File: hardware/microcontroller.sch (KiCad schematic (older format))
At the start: 10 parts, among them J1 Conn_02x05_Odd_Even, U1 ESP-WROOM-32

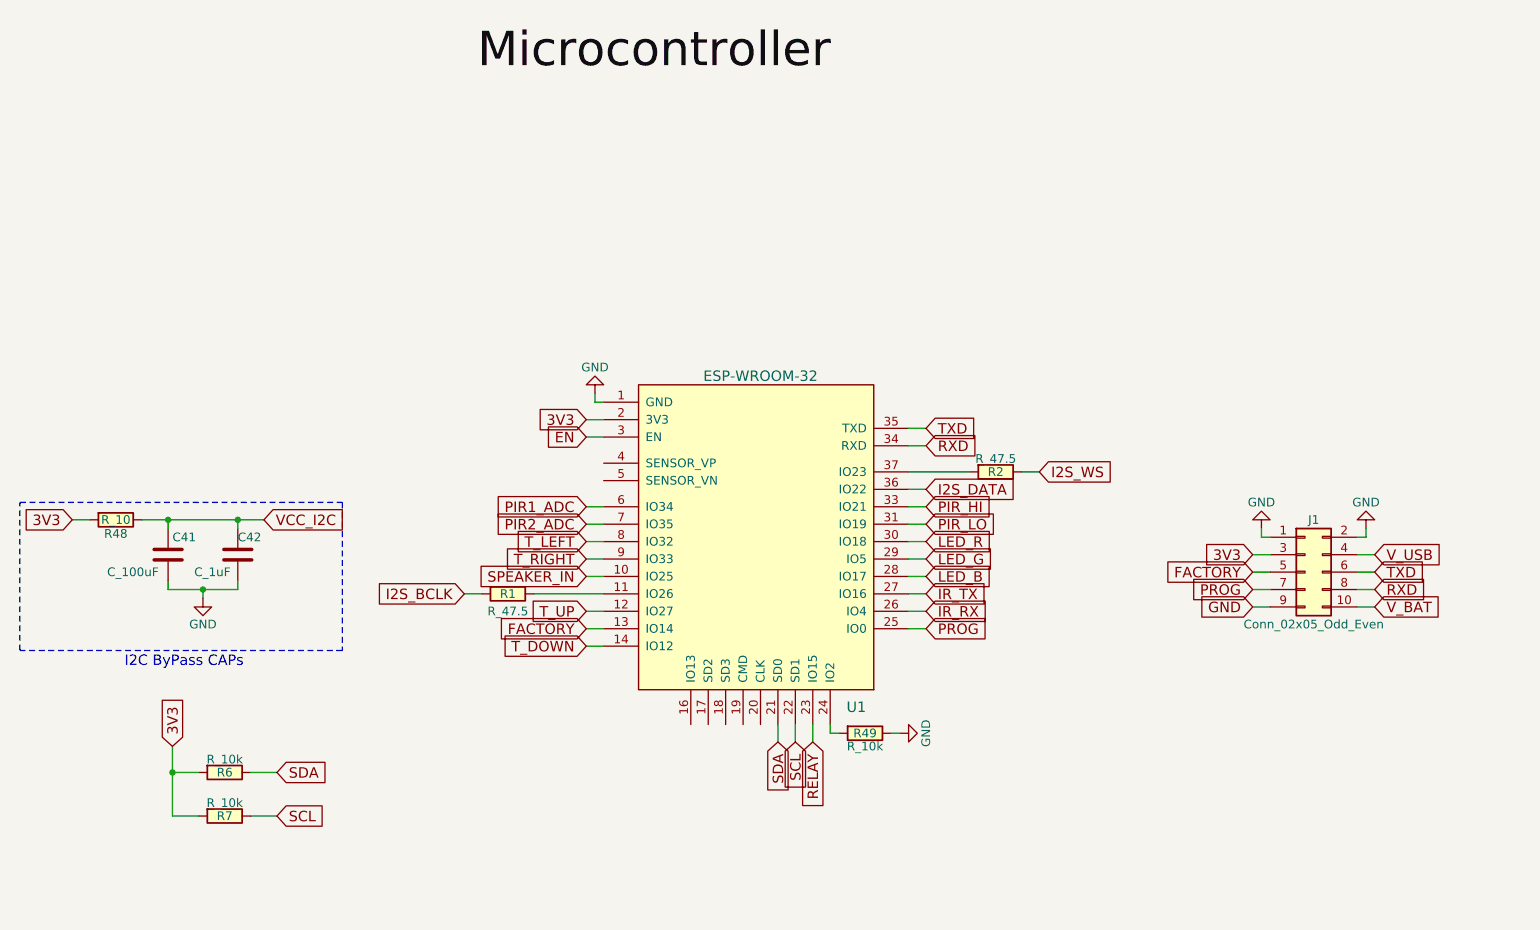
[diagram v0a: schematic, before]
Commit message: update
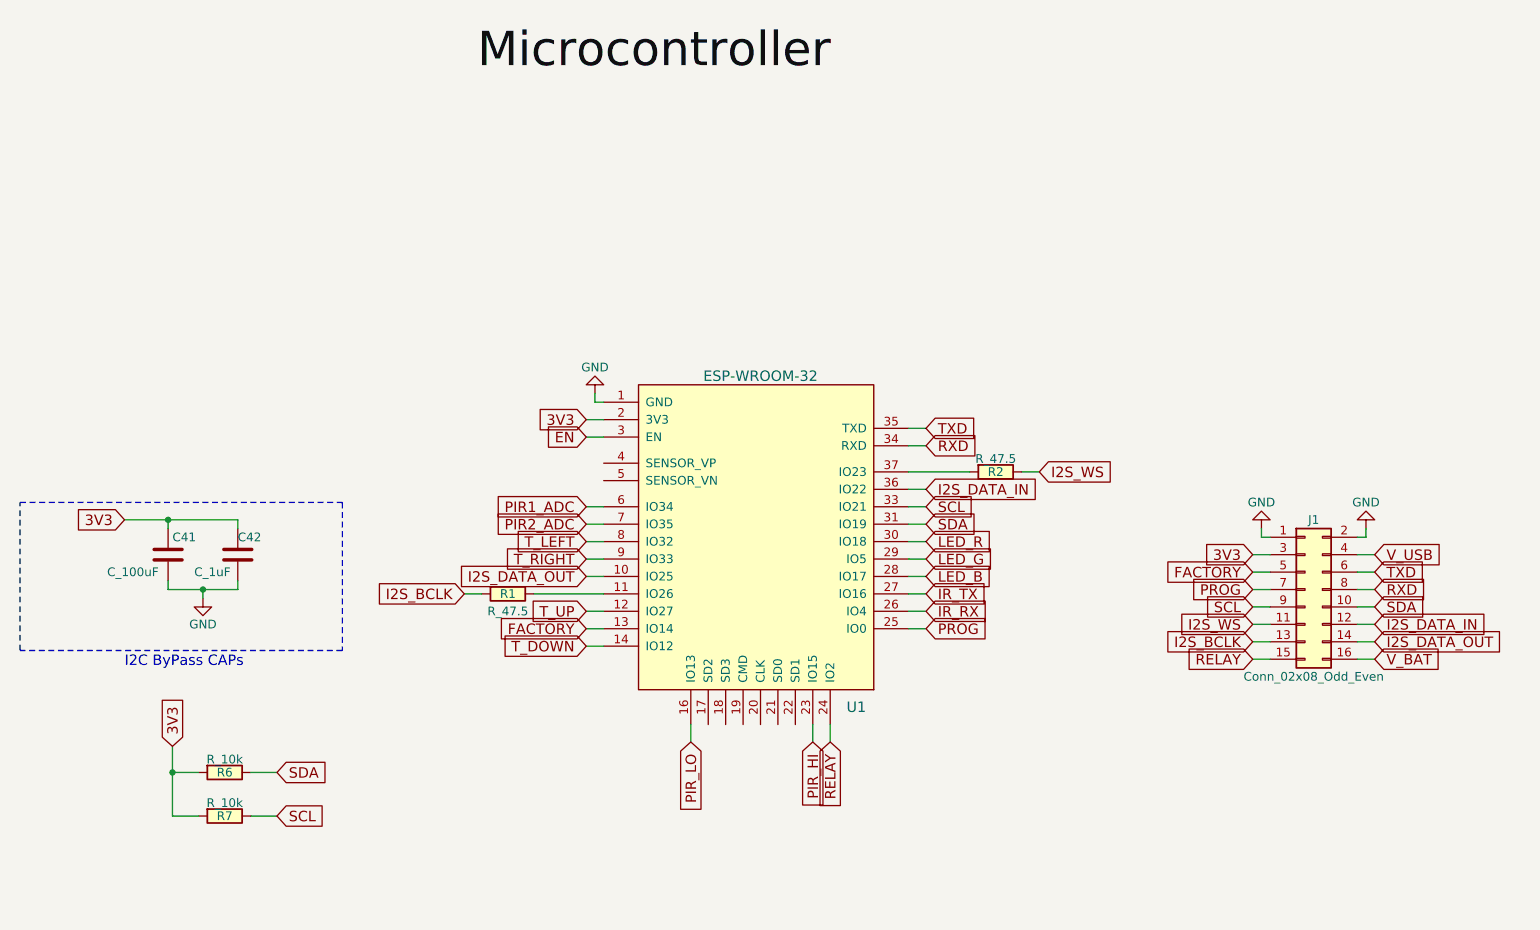
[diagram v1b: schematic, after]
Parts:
- removed J1: Conn_02x05_Odd_Even, Pin_Headers:Pin_Header_Straight_2x05_Pitch2.54mm, symbol Conn_02x05_Odd_Even
- removed R48: R_10, Resistors_SMD:R_0603, symbol R_10
- removed R49: R_10k, Resistors_SMD:R_0603, symbol R_10k
- added J1: Conn_02x08_Odd_Even, Pin_Headers:Pin_Header_Straight_2x08_Pitch2.54mm, symbol Conn_02x08_Odd_Even
- C41: footprint Capacitors_SMD:C_1206 -> Capacitors_SMD:C_1206_HandSoldering
- C42: footprint Capacitors_SMD:C_0603 -> Capacitors_SMD:C_0603_HandSoldering
- R1, R2, R6, R7: footprint Resistors_SMD:R_0603 -> Resistors_SMD:R_0603_HandSoldering
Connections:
- net VCC_I2C is gone; now on net 3V3: C41.1, C42.1
- net 3V3: now also J1.3 (Pin_3)
- net FACTORY: now also J1.5 (Pin_5)
- net GND: now also J1.1 (Pin_1), J1.2 (Pin_2)
- net I2S_BCLK: now also J1.13 (Pin_13)
- net I2S_WS: now also J1.11 (Pin_11)
- net PIR_HI: now also U1.23 (IO15); no longer U1.33 (IO21)
- net PIR_LO: now also U1.16 (IO13); no longer U1.31 (IO19)
- net PROG: now also J1.7 (Pin_7)
- net RELAY: now also U1.24 (IO2), J1.15 (Pin_15); no longer U1.23 (IO15)
- net RXD: now also J1.8 (Pin_8)
- net SCL: now also U1.33 (IO21), J1.9 (Pin_9); no longer U1.22 (SD1)
- net SDA: now also U1.31 (IO19), J1.10 (Pin_10); no longer U1.21 (SD0)
- net TXD: now also J1.6 (Pin_6)
- net V_BAT: now also J1.16 (Pin_16)
- net V_USB: now also J1.4 (Pin_4)
- net I2S_DATA renamed I2S_DATA_IN
- net I2S_DATA_IN: now also J1.12 (Pin_12)
- net SPEAKER_IN renamed I2S_DATA_OUT
- net I2S_DATA_OUT: now also J1.14 (Pin_14)

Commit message: update
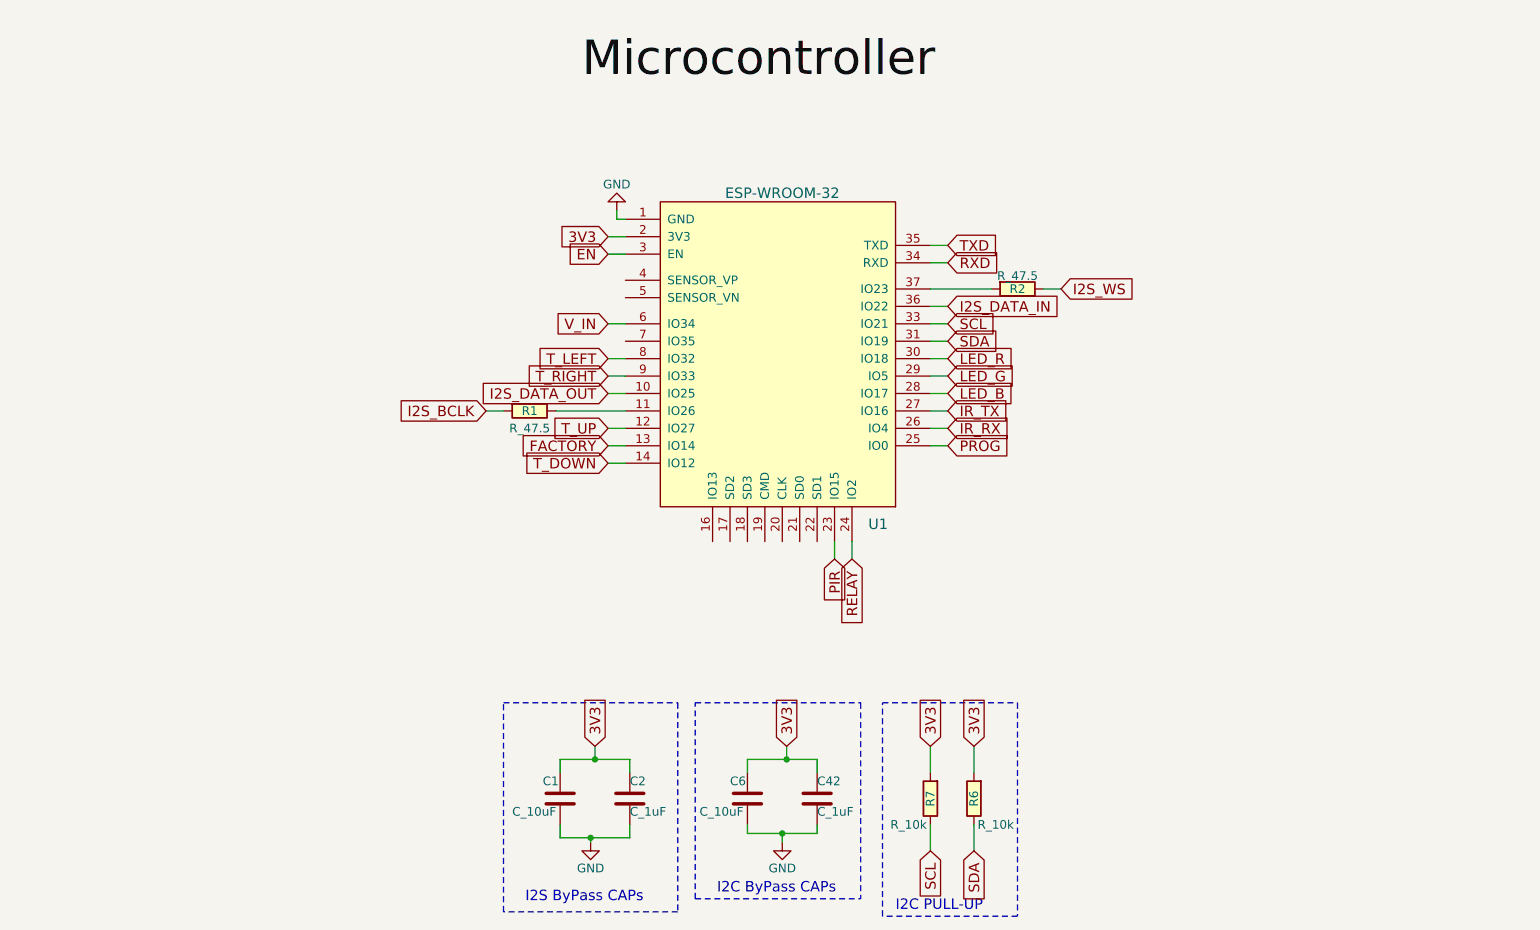
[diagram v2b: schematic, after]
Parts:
- removed C41: C_100uF, Capacitors_SMD:C_1206_HandSoldering, symbol C_100uF
- removed J1: Conn_02x08_Odd_Even, Pin_Headers:Pin_Header_Straight_2x08_Pitch2.54mm, symbol Conn_02x08_Odd_Even
- added C1, C6: C_10uF, Capacitors_SMD:C_0603_HandSoldering, symbol C_10uF
- added C2: C_1uF, Capacitors_SMD:C_0603_HandSoldering, symbol C_1uF
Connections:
- net 3V3: now also C1.1, C2.1, C6.1
- net GND: now also C1.2, C2.2, C6.2
- net PIR1_ADC renamed V_IN
- net PIR2_ADC: no longer names the net of U1.7 (IO35)
- net PIR_HI renamed PIR
- net PIR_LO: no longer names the net of U1.16 (IO13)
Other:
- note added: "I2C PULL-UP"
- note added: "I2S ByPass CAPs"
- moved on the sheet: C42, R1, R2, R6, R7, U1
